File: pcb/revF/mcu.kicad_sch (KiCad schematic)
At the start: 32 parts, among them CON4 JOYSTICK, CON5 KEYBOARD, CON6 MOUSE, J10 EXT JOYSTICK, J5 AVR JTAG, J6 AVR UART, U5 ATMEGA328-AU, U8 TXB0104PW, U9 DS1307Z+, Y1 32768Hz, Y2 16MHz

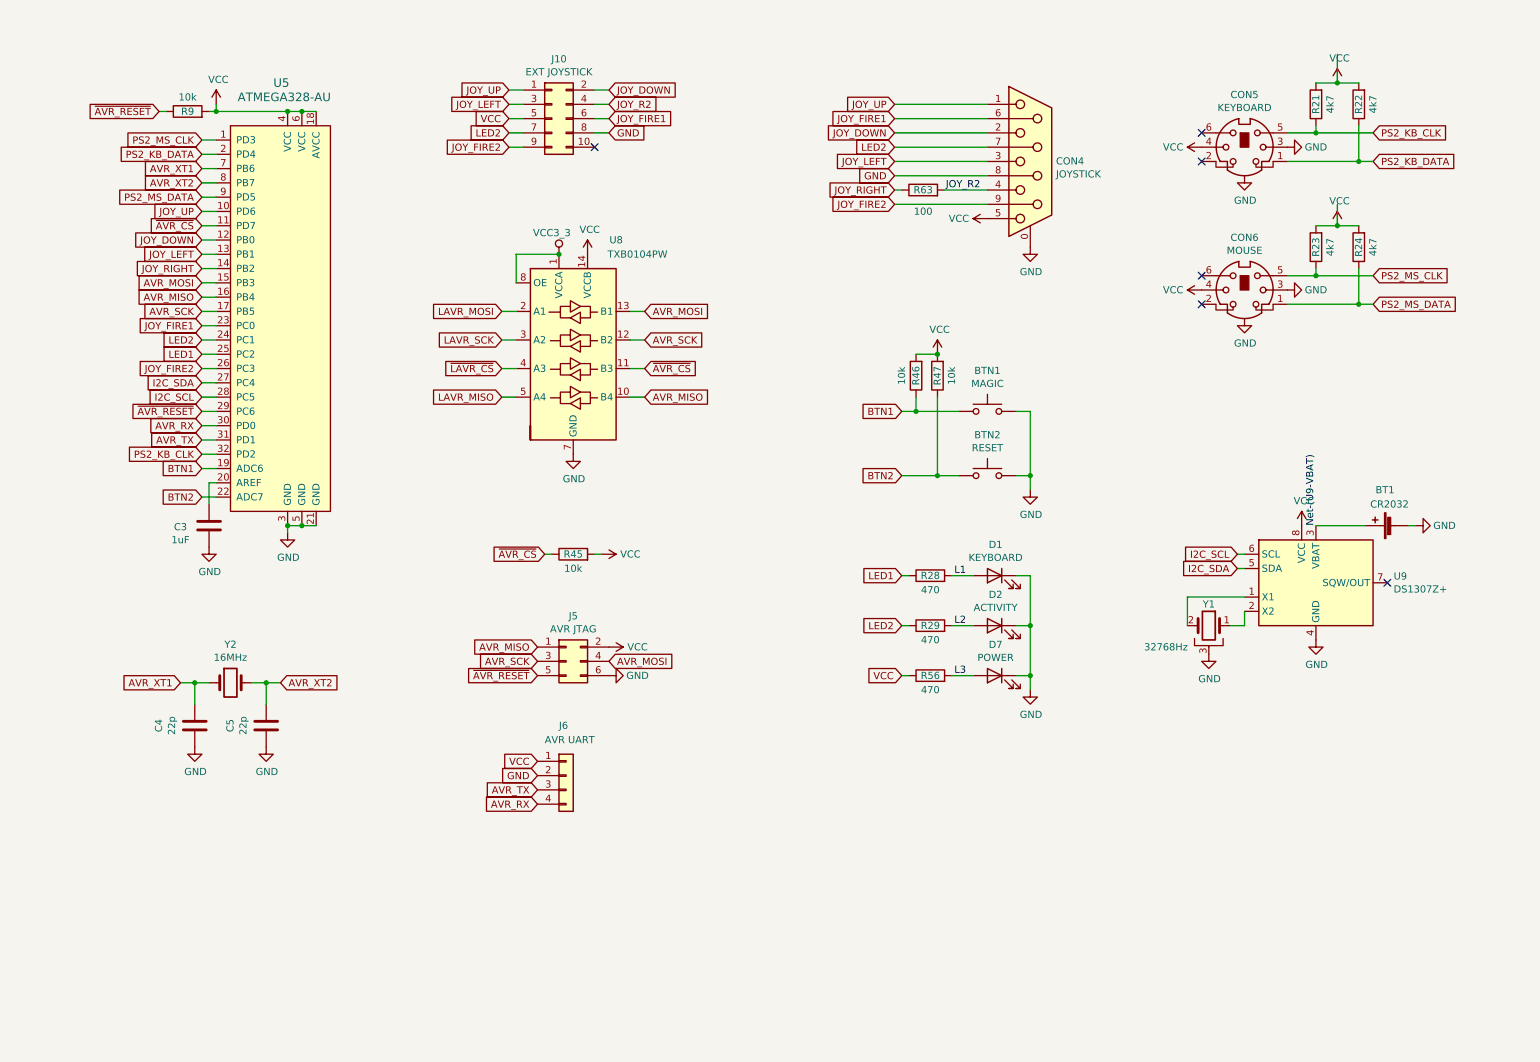
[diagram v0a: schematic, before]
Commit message: New schematics / revF
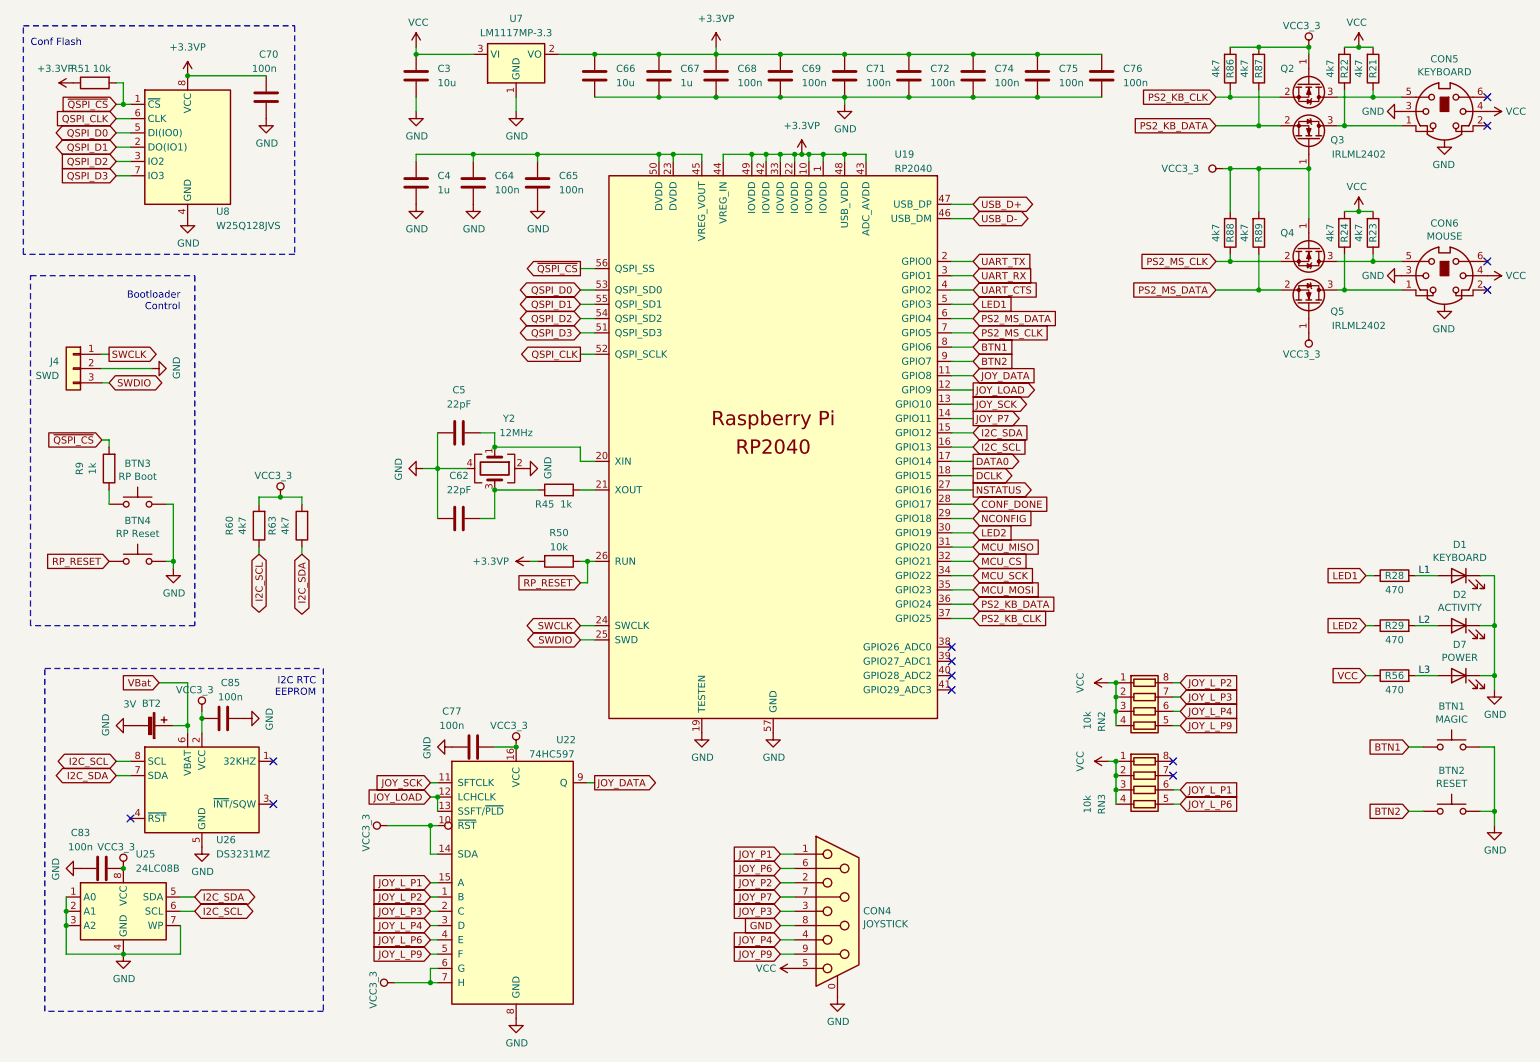
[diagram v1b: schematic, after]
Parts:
- removed BT1: CR2032, footprints:BAT_BS-7-BLUE, symbol Device:Battery_Cell
- removed J10: EXT JOYSTICK, Connector_PinHeader_2.54mm:PinHeader_2x05_P2.54mm_Vertical, symbol Connector_Generic:Conn_02x05_Odd_Even
- removed J5: AVR JTAG, Connector_IDC:IDC-Header_2x03_P2.54mm_Horizontal, symbol Connector_Generic:Conn_02x03_Odd_Even
- removed J6: AVR UART, Connector_PinHeader_2.54mm:PinHeader_1x04_P2.54mm_Vertical, symbol Connector_Generic:Conn_01x04
- removed R46, R47: 10k, Resistor_SMD:R_0805_2012Metric_Pad1.15x1.40mm_HandSolder, symbol Device:R
- removed U5: ATMEGA328-AU, Package_QFP:TQFP-32_7x7mm_P0.8mm, symbol dk_Embedded-Microcontrollers:ATMEGA328-AU
- removed U8: TXB0104PW, Package_SO:TSSOP-14_4.4x5mm_P0.65mm, symbol Logic_LevelTranslator:TXB0104PW
- removed U9: DS1307Z+, Package_SO:SOIC-8_3.9x4.9mm_P1.27mm, symbol Timer_RTC:DS1307Z+
- removed Y1: 32768Hz, Crystal:Crystal_AT310_D3.0mm_L10.0mm_Horizontal_1EP_style2, symbol Device:Crystal_GND3
- removed Y2: 16MHz, Crystal:Crystal_HC49-U_Vertical, symbol Device:Crystal
- added BT2: 3V, footprints:BAT_BS-7-BLUE, symbol Device:Battery_Cell
- added BTN3: RP Boot, footprints:SW_SPST_PTS810_handsoldering, symbol Switch:SW_Push
- added BTN4: RP Reset, footprints:SW_SPST_PTS810_handsoldering, symbol Switch:SW_Push
- added C62: 22pF, Capacitor_SMD:C_0805_2012Metric_Pad1.18x1.45mm_HandSolder, symbol Device:C
- added C64, C65, C68, C69, C70, C71, C72, C74, C75, C76, C77, C83, C85: 100n, Capacitor_SMD:C_0805_2012Metric_Pad1.18x1.45mm_HandSolder, symbol Device:C
- added C66: 10u, Capacitor_SMD:C_0805_2012Metric_Pad1.18x1.45mm_HandSolder, symbol Device:C
- added C67: 1u, Capacitor_SMD:C_0805_2012Metric_Pad1.18x1.45mm_HandSolder, symbol Device:C
- added J4: SWD, Connector_PinHeader_2.54mm:PinHeader_1x03_P2.54mm_Vertical, symbol Connector_Generic:Conn_01x03
- added Q2, Q3, Q4, Q5: IRLML2402, Package_TO_SOT_SMD:SOT-23, symbol Transistor_FET:IRLML0030
- added R50, R51: 10k, Resistor_SMD:R_0805_2012Metric_Pad1.20x1.40mm_HandSolder, symbol Device:R
- added R60: 4k7, Resistor_SMD:R_0805_2012Metric_Pad1.20x1.40mm_HandSolder, symbol Device:R
- added R86, R87, R88, R89: 4k7, Resistor_SMD:R_0805_2012Metric_Pad1.15x1.40mm_HandSolder, symbol Device:R
- added RN2, RN3: 10k, Resistor_SMD:R_Array_Convex_4x0603, symbol Device:R_Pack04
- added U19: RP2040, RP2040_minimal:RP2040-QFN-56, symbol MCU_RaspberryPi_RP2040:RP2040
- added U22: 74HC597, Package_SO:SO-16_3.9x9.9mm_P1.27mm, symbol retro:74hc597
- added U25: 24LC08B, Package_SO:SO-8_3.9x4.9mm_P1.27mm, symbol Memory_EEPROM:24LC08
- added U26: DS3231MZ, Package_SO:SOIC-8_3.9x4.9mm_P1.27mm, symbol Timer_RTC:DS3231MZ
- added U7: LM1117MP-3.3, Package_TO_SOT_SMD:SOT-223-3_TabPin2, symbol Regulator_Linear:LM1117MP-3.3
- added U8: W25Q128JVS, Package_SO:SOIC-8_5.23x5.23mm_P1.27mm, symbol Memory_Flash:W25Q128JVS
- added Y2: 12MHz, Crystal:Crystal_SMD_3225-4Pin_3.2x2.5mm_HandSoldering, symbol Device:Crystal_GND24
- C3: value 1uF -> 10u; footprint Capacitor_SMD:C_0805_2012Metric_Pad1.15x1.40mm_HandSolder -> Capacitor_SMD:C_0805_2012Metric_Pad1.18x1.45mm_HandSolder
- C4: value 22p -> 1u; footprint Capacitor_SMD:C_0805_2012Metric_Pad1.15x1.40mm_HandSolder -> Capacitor_SMD:C_0805_2012Metric_Pad1.18x1.45mm_HandSolder
- C5: value 22p -> 22pF; footprint Capacitor_SMD:C_0805_2012Metric_Pad1.15x1.40mm_HandSolder -> Capacitor_SMD:C_0805_2012Metric_Pad1.18x1.45mm_HandSolder
- R45, R9: value 10k -> 1k; footprint Resistor_SMD:R_0805_2012Metric_Pad1.15x1.40mm_HandSolder -> Resistor_SMD:R_0805_2012Metric_Pad1.20x1.40mm_HandSolder
- R63: value 100 -> 4k7; footprint Resistor_SMD:R_0805_2012Metric_Pad1.15x1.40mm_HandSolder -> Resistor_SMD:R_0805_2012Metric_Pad1.20x1.40mm_HandSolder
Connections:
- net AVR_XT1 is gone; now on net GND: C4.2
- net AVR_XT2 is gone; now on net GND: C5.2
- net JOY_RIGHT is gone; now on net I2C_SDA: R63.1
- net BTN1: now also U19.8 (GPIO6)
- net BTN2: now also U19.9 (GPIO7)
- net GND: now also C3.2, BT2.2 (-), BTN3.2, BTN4.2, C62.2, C64.2, C65.2, C66.2, C67.2, C68.2, C69.2, C70.1, C71.2, C72.2, C74.2, C75.2, C76.2, C77.2, C83.2, C85.2, J4.2 (Pin_2), U19.19 (TESTEN), U19.57 (GND), U22.8 (GND), U25.1 (A0), U25.2 (A1), U25.3 (A2), U25.4 (GND), U25.7 (WP), U26.5 (GND), U7.1 (GND), U8.4 (GND), Y2.2, Y2.4; no longer C3.1, C4.1, C5.1
- net I2C_SCL: now also R60.1, U19.16 (GPIO13), U25.6 (SCL), U26.8 (SCL)
- net I2C_SDA: now also U19.15 (GPIO12), U25.5 (SDA), U26.7 (SDA)
- net LED1: now also U19.5 (GPIO3)
- net LED2: now also U19.30 (GPIO19); no longer CON4.7
- net PS2_KB_CLK: now also Q2.2 (S), R86.1, U19.37 (GPIO25); no longer CON5.5, R21.1
- net PS2_KB_DATA: now also Q3.2 (S), R87.1, U19.36 (GPIO24); no longer CON5.1, R22.1
- net PS2_MS_CLK: now also Q4.2 (S), R88.1, U19.7 (GPIO5); no longer CON6.5, R23.1
- net PS2_MS_DATA: now also Q5.2 (S), R89.1, U19.6 (GPIO4); no longer CON6.1, R24.1
- net VCC: now also C3.1, RN2.1 (R1.1), RN2.2 (R2.1), RN2.3 (R3.1), RN2.4 (R4.1), RN3.1 (R1.1), RN3.2 (R2.1), RN3.3 (R3.1), RN3.4 (R4.1), U7.3 (VI); no longer R45.2, R9.2
- net VCC3_3: now also R63.2, C77.1, C83.1, C85.1, Q2.1 (G), Q3.1 (G), Q4.1 (G), Q5.1 (G), R60.2, R86.2, R87.2, R88.2, R89.2, U22.10 (~{RST}), U22.14 (SDA), U22.16 (VCC), U22.6 (G), U22.7 (H), U25.8 (VCC), U26.2 (VCC)
- net JOY_DOWN renamed JOY_P2
- net JOY_FIRE1 renamed JOY_P6
- net JOY_FIRE2 renamed JOY_P9
- net JOY_LEFT renamed JOY_P3
- net JOY_R2 renamed JOY_P4
- net JOY_P4: no longer R63.2
- net JOY_UP renamed JOY_P1
- net ~{AVR_CS}: no longer names the net of R45.1
- net ~{AVR_CS}: now also C62.1, Y2.3
- net ~{AVR_RESET}: no longer names the net of R9.1
- net ~{AVR_RESET}: now also BTN3.1
- new net: CON6.1, Q5.3 (D), R24.1
- new net: CON5.1, Q3.3 (D), R22.1
- new net: C5.1, U19.20 (XIN), Y2.1
- new net: CON5.5, Q2.3 (D), R21.1
- new net: C4.1, C64.1, C65.1, U19.23 (DVDD), U19.45 (VREG_VOUT), U19.50 (DVDD)
- new net: CON6.5, Q4.3 (D), R23.1
- new net: R45.2, U19.21 (XOUT)
- new net +3.3VP: C66.1, C67.1, C68.1, C69.1, C70.2, C71.1, C72.1, C74.1, C75.1, C76.1, R50.2, R51.1, U19.1 (IOVDD), U19.10 (IOVDD), U19.22 (IOVDD), U19.33 (IOVDD), U19.42 (IOVDD), U19.43 (ADC_AVDD), U19.44 (VREG_IN), U19.48 (USB_VDD), U19.49 (IOVDD), U7.2 (VO), U8.8 (VCC)
- new net CONF_DONE: U19.28 (GPIO17)
- new net DATA0: U19.17 (GPIO14)
- new net DCLK: U19.18 (GPIO15)
- new net JOY_DATA: U19.11 (GPIO8), U22.9 (Q)
- new net JOY_LOAD: U19.12 (GPIO9), U22.12 (LCHCLK), U22.13 (SSFT/~{PLD})
- new net JOY_L_P1: RN3.6 (R3.2), U22.15 (A)
- new net JOY_L_P2: RN2.8 (R1.2), U22.1 (B)
- new net JOY_L_P3: RN2.7 (R2.2), U22.2 (C)
- new net JOY_L_P4: RN2.6 (R3.2), U22.3 (D)
- new net JOY_L_P6: RN3.5 (R4.2), U22.4 (E)
- new net JOY_L_P9: RN2.5 (R4.2), U22.5 (F)
- new net JOY_P7: CON4.7, U19.14 (GPIO11)
- new net JOY_SCK: U19.13 (GPIO10), U22.11 (SFTCLK)
- new net MCU_CS: U19.32 (GPIO21)
- new net MCU_MISO: U19.31 (GPIO20)
- new net MCU_MOSI: U19.35 (GPIO23)
- new net MCU_SCK: U19.34 (GPIO22)
- new net NCONFIG: U19.29 (GPIO18)
- new net NSTATUS: U19.27 (GPIO16)
- new net QSPI_CLK: U19.52 (QSPI_SCLK), U8.6 (CLK)
- new net QSPI_D0: U19.53 (QSPI_SD0), U8.5 (DI(IO0))
- new net QSPI_D1: U19.55 (QSPI_SD1), U8.2 (DO(IO1))
- new net QSPI_D2: U19.54 (QSPI_SD2), U8.3 (IO2)
- new net QSPI_D3: U19.51 (QSPI_SD3), U8.7 (IO3)
- new net RP_RESET: BTN4.1, R50.1, U19.26 (RUN)
- new net SWCLK: J4.1 (Pin_1), U19.24 (SWCLK)
- new net SWDIO: J4.3 (Pin_3), U19.25 (SWD)
- new net UART_CTS: U19.4 (GPIO2)
- new net UART_RX: U19.3 (GPIO1)
- new net UART_TX: U19.2 (GPIO0)
- new net USB_D+: U19.47 (USB_DP)
- new net USB_D-: U19.46 (USB_DM)
- new net VBat: BT2.1 (+), U26.6 (VBAT)
- new net ~{QSPI_CS}: R51.2, R9.2, U19.56 (QSPI_SS), U8.1 (~{CS})
- no-connect marks 6 -> 13
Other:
- note added: "Bootloader Control"
- note added: "Conf Flash"
- note added: "I2C RTC EEPROM"
- moved on the sheet: BTN1, BTN2, CON4, CON5, CON6, D1, D2, D7, R21, R22, R23, R24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
